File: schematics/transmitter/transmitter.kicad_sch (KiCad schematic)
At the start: 30 parts, among them J1 Program, J2 Debug, Q2 2N7000, SW1 Power, SW2 ~{MCLR}, U2 NRF24L01_Breakout, U3 AMS1117-3.3, U4 PIC32MX170F256B

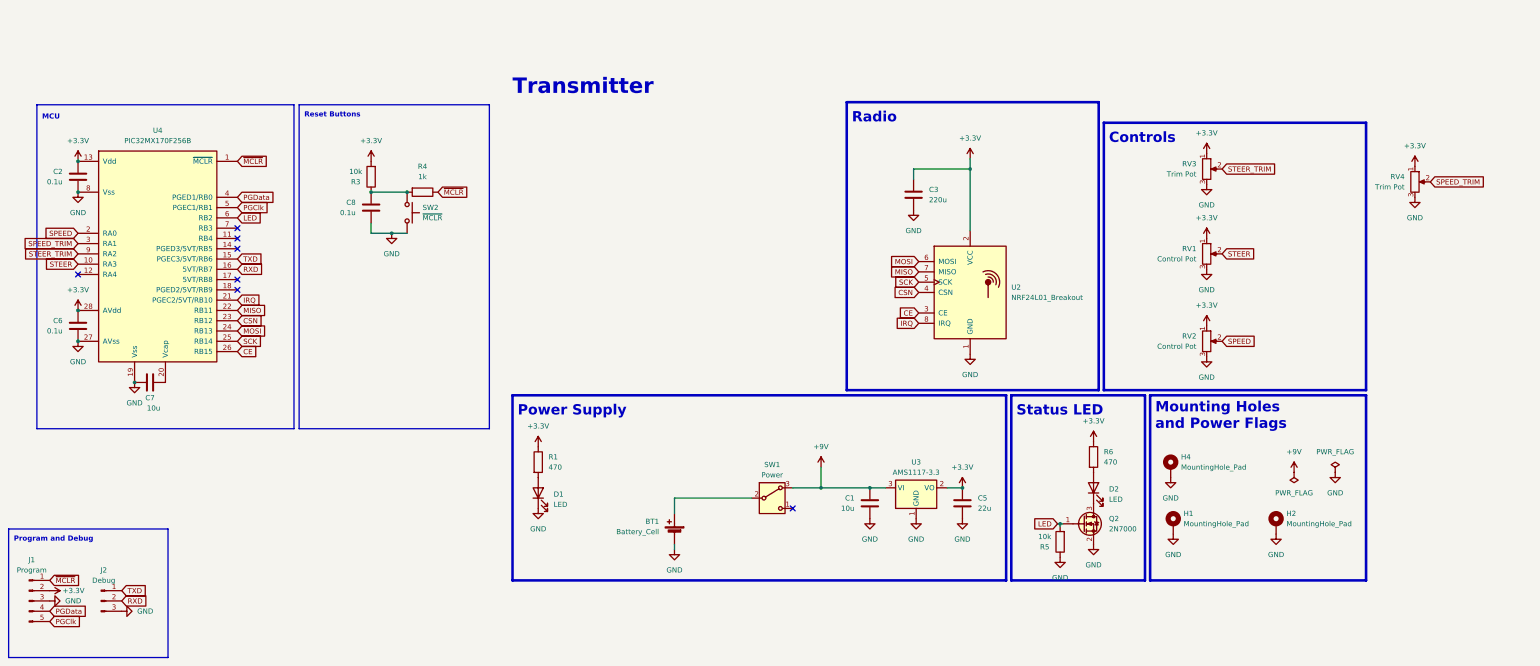
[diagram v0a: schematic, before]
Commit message: Update
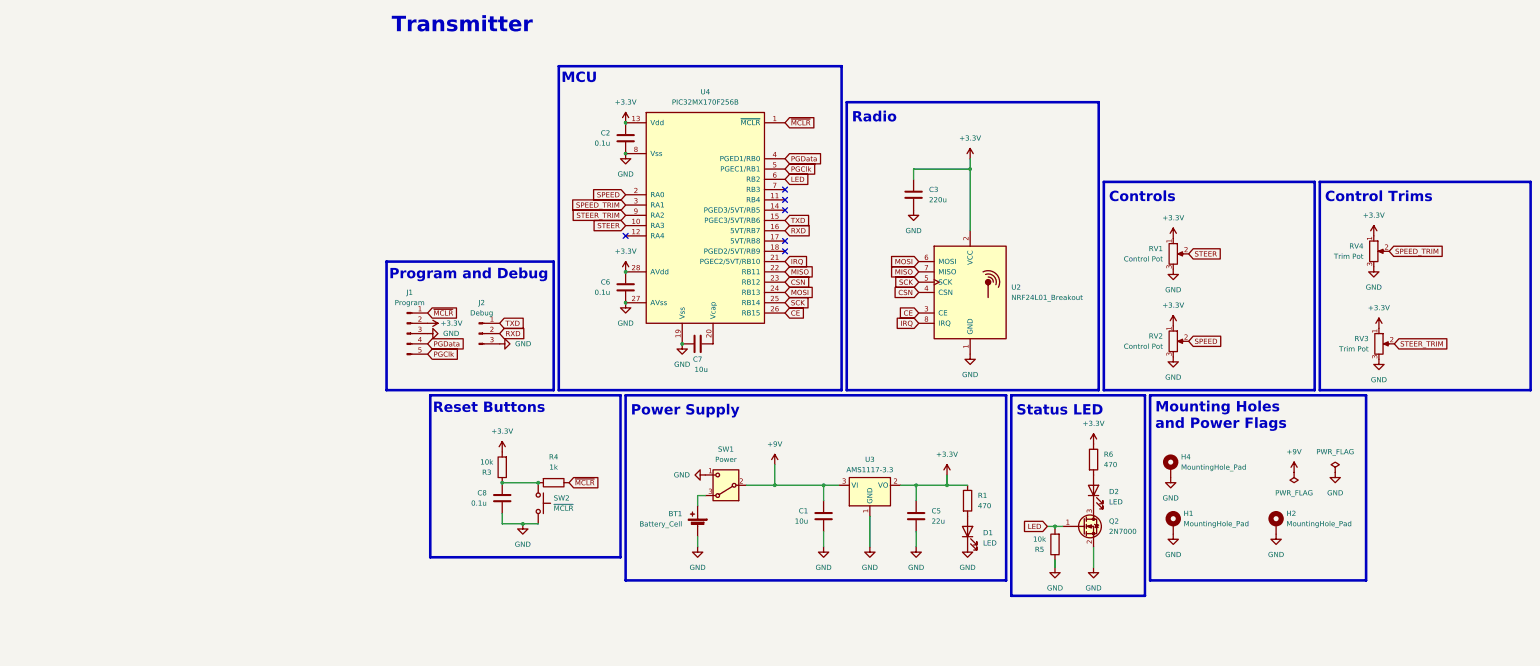
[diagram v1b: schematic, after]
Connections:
- net +9V: now also SW1.2 (B); no longer SW1.3 (A)
- net GND: now also SW1.1 (C)
- net at BT1.1 (+): now also SW1.3 (A); no longer SW1.2 (B)
- no-connect marks 7 -> 6
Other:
- note added: "Control Trims"
- moved on the sheet: BT1, C1, C2, C5, C6, C7, C8, D1, D2, J1, J2, Q2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
